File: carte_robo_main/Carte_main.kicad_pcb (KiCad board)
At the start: 2 copper layers, 45 x 50.5 mm, 13 parts, among them J1 Conn_01x18_Pin, J2 Conn_01x18_Pin, J3 Conn_01x02_Socket, J4 Conn_01x05_Socket

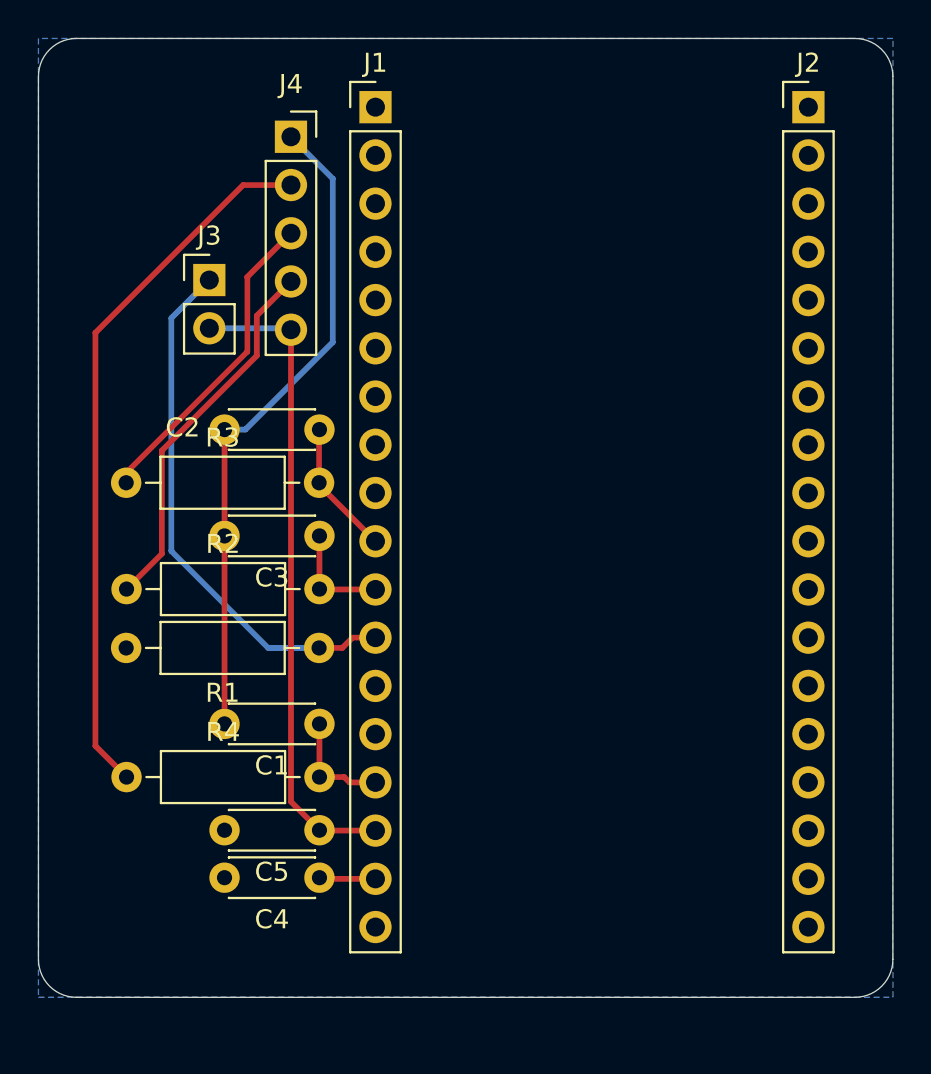
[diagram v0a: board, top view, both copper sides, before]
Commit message: last update
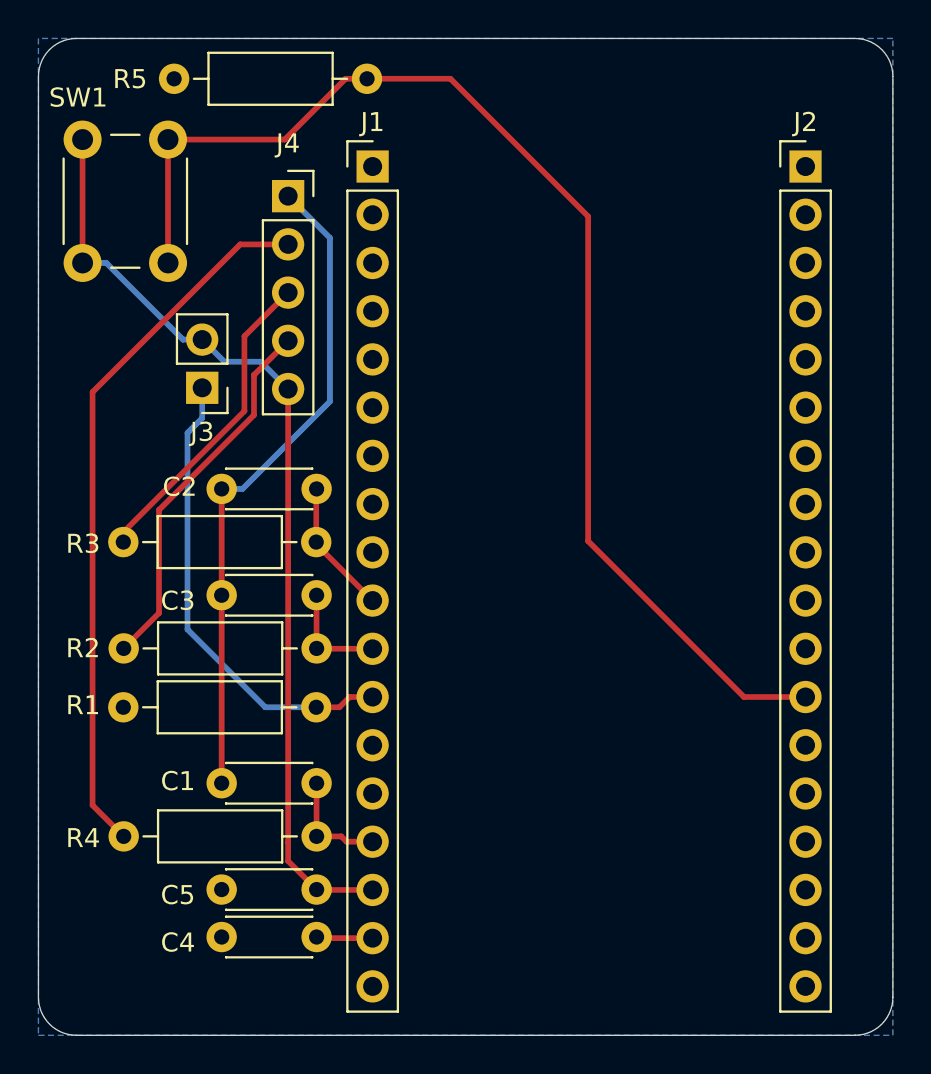
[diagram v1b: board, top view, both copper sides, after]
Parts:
- added R5: 100k, Resistor_THT:R_Axial_DIN0207_L6.3mm_D2.5mm_P10.16mm_Horizontal, F.Cu at (123.1, 74.1)
- added SW1: SW_Push, Button_Switch_THT:SW_PUSH_6mm_H5mm, F.Cu at (118.3, 83.8)
- moved J3 5.69 mm to (124.6, 90.4), turned to 180 degrees
- moved C1 3.13 mm to (130.7, 111.2)
- moved C2 3.13 mm to (130.7, 95.7)
- moved C3 3.13 mm to (130.7, 101.3)
- moved C4 3.13 mm to (130.7, 119.3)
- moved C5 3.13 mm to (130.7, 116.8)
- moved J1 3.13 mm to (133.6, 78.7)
- moved J2 3.13 mm to (156.4, 78.7)
- moved J4 3.13 mm to (129.2, 80.3)
- moved R1 3.13 mm to (130.6, 107.2)
- moved R2 3.13 mm to (120.5, 104.1)
- moved R3 3.13 mm to (120.5, 98.5)
- moved R4 3.13 mm to (120.5, 114.0)
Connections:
- J2 pad 12: unconnected-(J2-Pin_12-Pad12) -> Net-(J2-Pin_12)
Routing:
- net Net-(J2-Pin_12): track 0.00 -> 64.9 mm
- net /+3.3V: track 34.3 -> 50.0 mm
- net /39: track 28.2 -> 24.7 mm
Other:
- board size 45 x 50.5 mm -> 45 x 52.5 mm
